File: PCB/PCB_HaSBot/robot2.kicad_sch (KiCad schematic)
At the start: 21 parts, among them J1 Conn_01x04, J10 Conn_01x08, J11 Conn_01x08, J12 Conn_01x06, J2 Conn_01x04, J3 Conn_01x04, J4 Conn_01x04, J5 Conn_01x04, J6 Conn_01x04, J7 Conn_01x04, J8 Screw_Terminal_01x02, J9 Conn_01x10, M1 Motor_Servo, U3 L7805

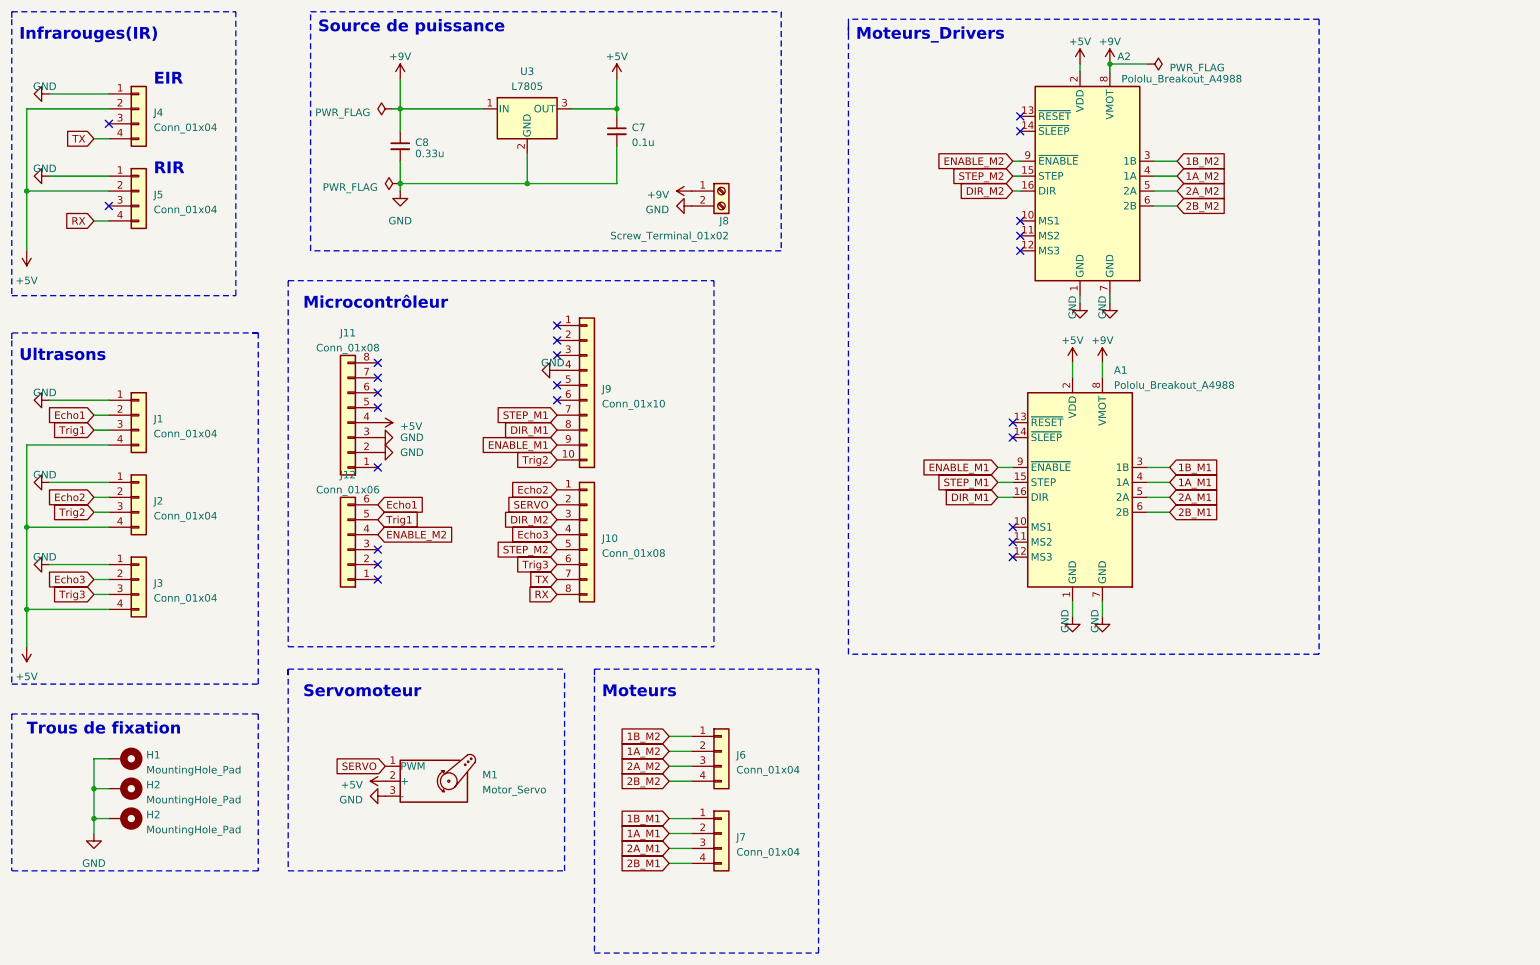
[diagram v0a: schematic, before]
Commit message: Version finale du pcb
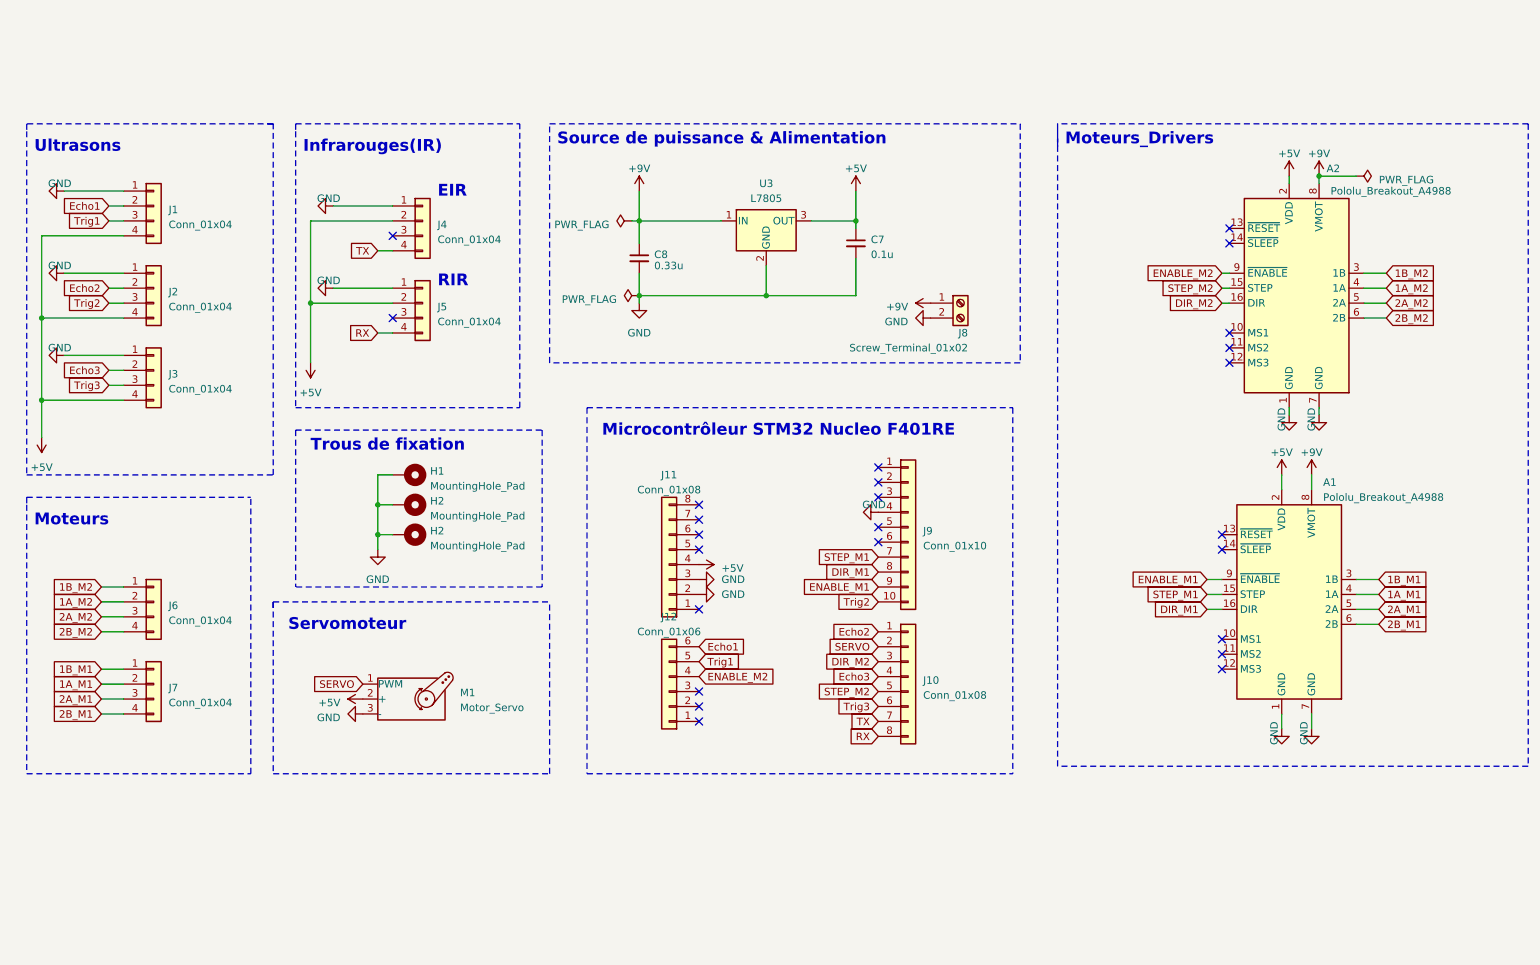
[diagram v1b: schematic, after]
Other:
- note added: "Microcontrôleur STM32 Nucleo F401RE"
- note added: "Source de puissance & Alimentation"
- note removed: "Microcontrôleur"
- note removed: "Source de puissance"
- moved on the sheet: A1, A2, C7, C8, H1, H2, J1, J10, J11, J12, J2, J3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
